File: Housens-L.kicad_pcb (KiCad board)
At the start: 4 copper layers, 50 x 50 mm, 45 parts, among them J1 JTAG/SWD, J2 USB_C_2.0, Q1 DMC3071LVT, SW1 RESET, SW2 USER, U1 MCP1603, U2 BME280, U3 OPT3005, U4 STM32WB55CGUx, Y1 32MHz, Y2 32.768kHz

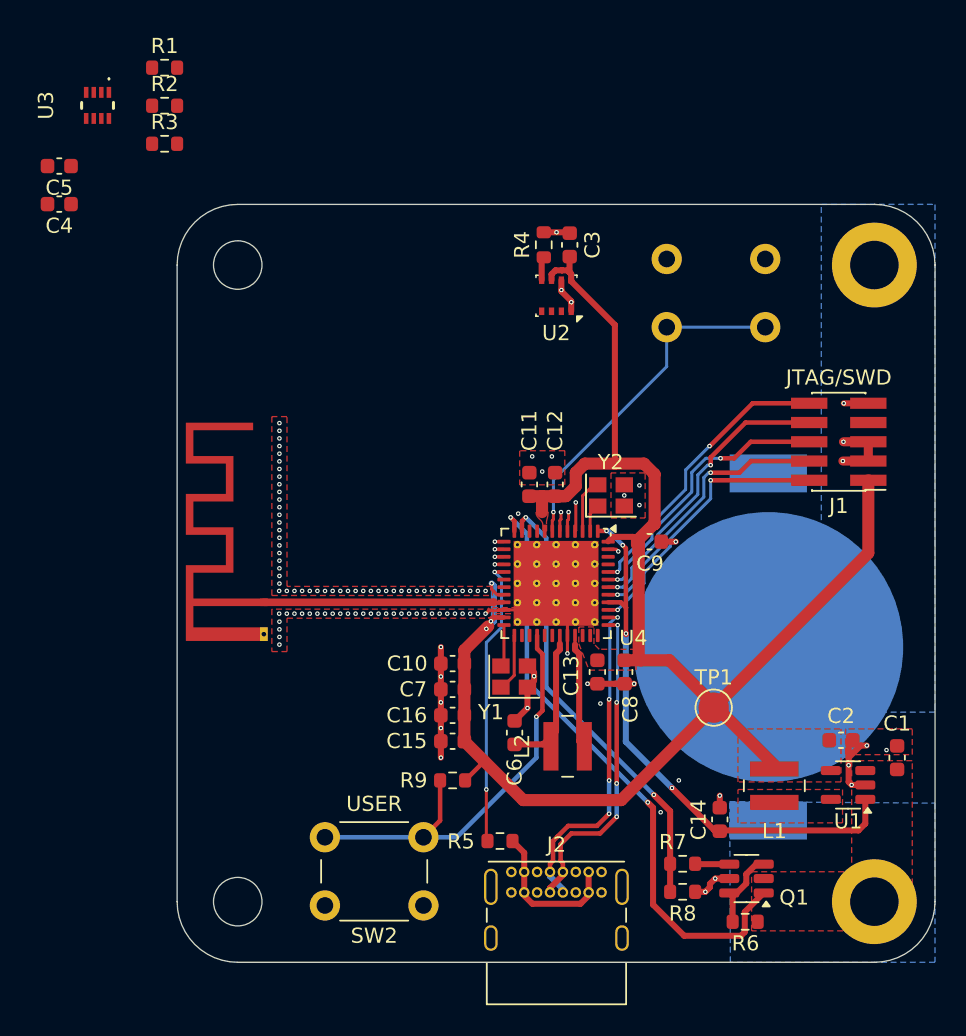
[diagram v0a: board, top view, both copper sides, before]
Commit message: Layout I2C
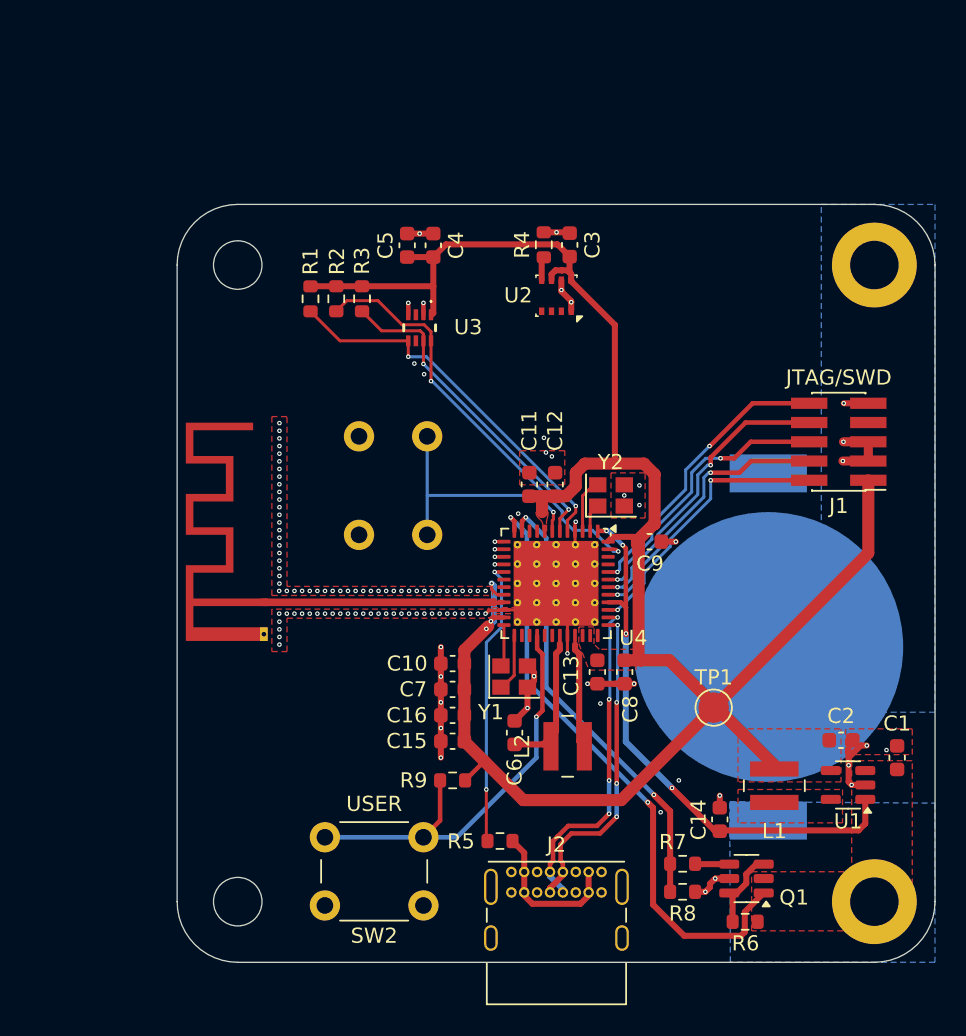
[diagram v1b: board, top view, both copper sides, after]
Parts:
- moved SW1 29.2 mm to (72.0, 95.3), turned to -90 degrees
- moved U3 25.8 mm to (76.0, 88.1)
- moved C4 24.8 mm to (76.9, 82.7), turned to 90 degrees
- moved C5 23.5 mm to (75.2, 82.7), turned to 90 degrees
- moved R1 18.0 mm to (68.8, 86.2), turned to -90 degrees
- moved R2 17.0 mm to (70.5, 86.2), turned to -90 degrees
- moved R3 16.6 mm to (72.2, 86.2), turned to -90 degrees
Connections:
- U4 pad 4: /BOOT0 -> GND
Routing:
- net /I2C1_SDA: track 0.73 -> 28.7 mm, vias 1 -> 2
- net /I2C1_SCL: track 1.29 -> 25.3 mm, vias 1 -> 2
- net +1V8: track 113.7 -> 137.0 mm
- net /OPT_INT: track 1.29 -> 21.9 mm, vias 1 -> 2
- net Net-(U4-NRST): track 23.1 -> 16.6 mm
- net GND: track 46.8 -> 51.7 mm, vias 116 -> 122
- net /BOOT0: track 1.92 -> 0.00 mm, vias 1 -> 0
